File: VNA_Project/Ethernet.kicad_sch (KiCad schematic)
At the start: 0 parts

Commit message: minor changes eth
minor changes eth
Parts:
- added J1001: RJ45_Wuerth_7499010211A, Connector_RJ:RJ45_Wuerth_7499010211A_Horizontal, symbol Connector:RJ45_Wuerth_7499010211A
- added U1001: DP83848C, Package_QFP:LQFP-48_7x7mm_P0.5mm, symbol Interface_Ethernet:DP83848C
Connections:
- new net +3.3V: U1001.32 (IOVDD33), U1001.48 (IOVDD33)
- new net +3.3VA: U1001.22 (AVDD33)
- new net ETH_CRS_DV: U1001.40 (CRS/CRS_DV/LED_CFG)
- new net ETH_MDIO: U1001.30 (MDIO)
- new net ETH_RXD0: U1001.43 (RXD_0/PHY_AD1)
- new net ETH_RXD1: U1001.44 (RXD_1/PHY_AD2)
- new net ETH_RX_CLK: U1001.38 (RX_CLK)
- new net ETH_TXD0: U1001.3 (TXD_0)
- new net ETH_TXD1: U1001.4 (TXD_1)
- new net ETH_TX_EN: U1001.2 (TX_EN)
- new net GND: U1001.15 (AGND), U1001.19 (AGND), U1001.35 (IOGND), U1001.36 (DGND), U1001.47 (IOGND)
- new net NRST: U1001.29 (~{RESET})

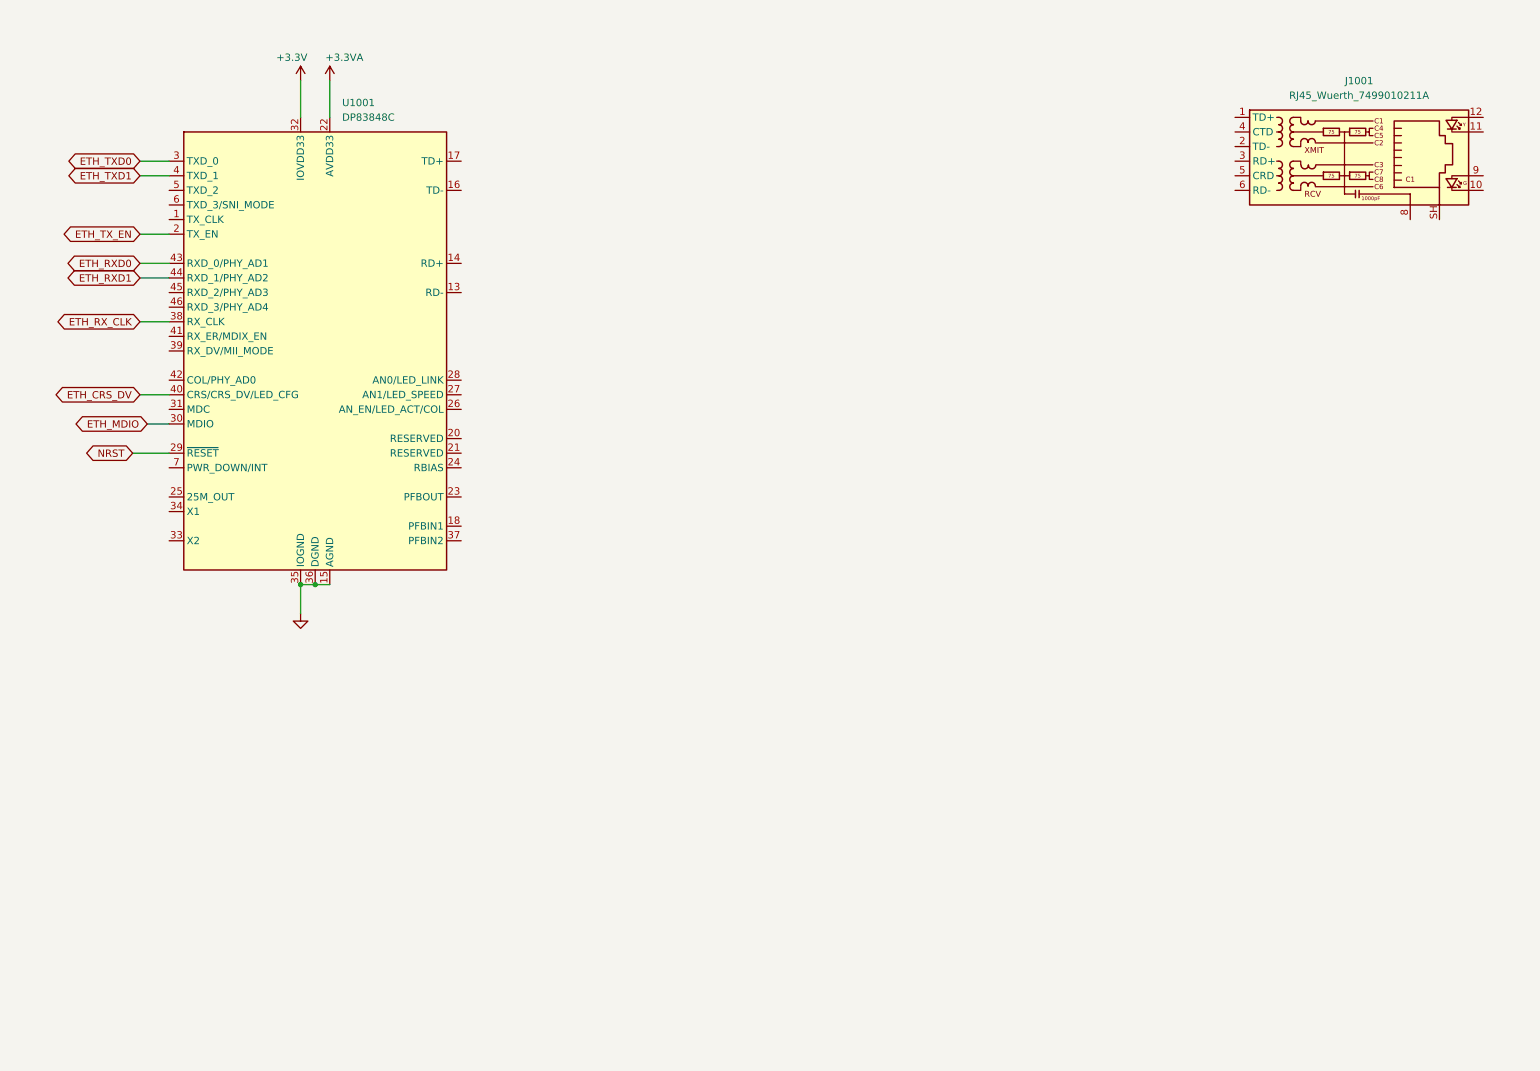
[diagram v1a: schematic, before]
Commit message: eth
eth
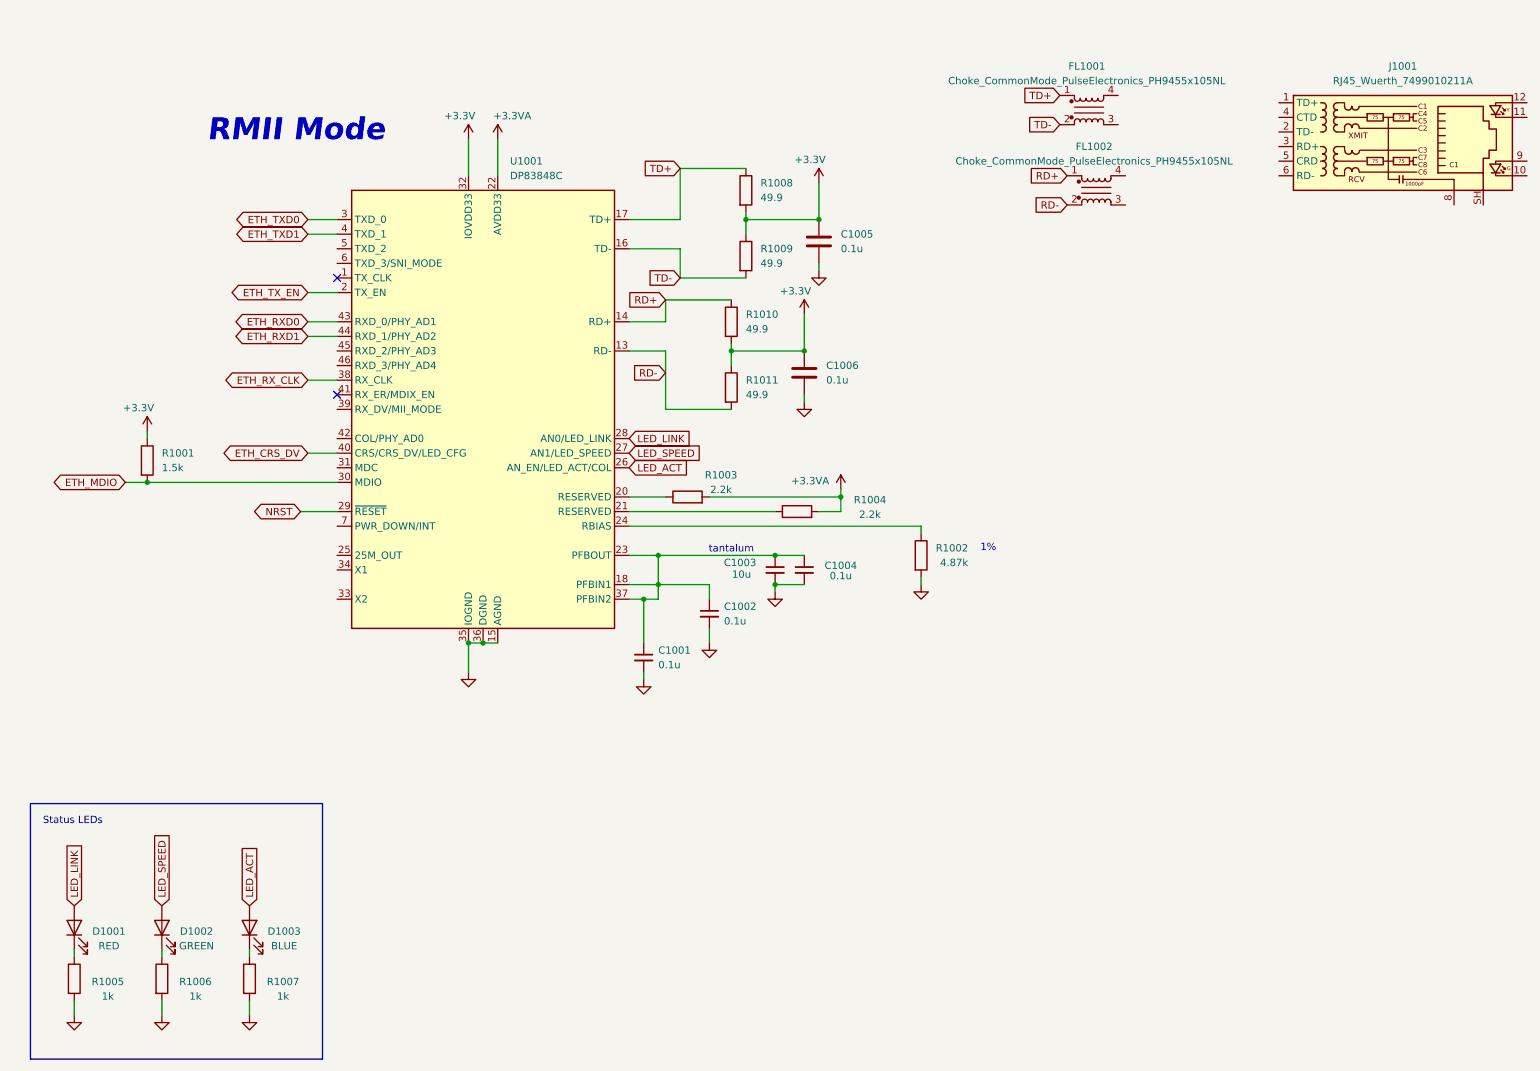
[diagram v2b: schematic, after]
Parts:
- added C1001, C1002, C1004: 0.1u, symbol Device:C_Small
- added C1003: 10u, symbol Device:C_Small
- added C1005, C1006: 0.1u, symbol Device:C
- added D1001: RED, symbol Device:LED
- added D1002: GREEN, symbol Device:LED
- added D1003: BLUE, symbol Device:LED
- added FL1001, FL1002: Choke_CommonMode_PulseElectronics_PH9455x105NL, Inductor_THT:L_CommonMode_PulseElectronics_PH9455x105NL_1, symbol Filter:Choke_CommonMode_PulseElectronics_PH9455x105NL
- added R1001: 1.5k, symbol Device:R
- added R1002: 4.87k, symbol Device:R
- added R1003, R1004: 2.2k, symbol Device:R
- added R1005, R1006, R1007: 1k, symbol Device:R
- added R1008, R1009, R1010, R1011: 49.9, symbol Device:R
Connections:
- net +3.3V: now also C1005.1, C1006.1, R1001.1, R1008.2, R1009.1, R1010.2, R1011.1
- net +3.3VA: now also R1003.2, R1004.2
- net ETH_MDIO: now also R1001.2
- net GND: now also C1001.2, C1002.2, C1003.2, C1004.2, C1005.2, C1006.2, R1002.2, R1005.2, R1006.2, R1007.2
- net RD-: now reaches U1001.13 (RD-)
- net RD-: now also FL1002.2, R1011.2
- net RD+: now reaches U1001.14 (RD+)
- net RD+: now also FL1002.1, R1010.1
- net TD-: now reaches U1001.16 (TD-)
- net TD-: now also FL1001.2, R1009.2
- net TD+: now reaches U1001.17 (TD+)
- net TD+: now also FL1001.1, R1008.1
- net at U1001.18 (PFBIN1): now also U1001.23 (PFBOUT), U1001.37 (PFBIN2), C1001.1, C1002.1, C1003.1, C1004.1
- net at U1001.20 (RESERVED): now also R1003.1
- net at U1001.21 (RESERVED): now also R1004.1
- net at U1001.24 (RBIAS): now also R1002.1
- net LED_ACT: now reaches U1001.26 (AN_EN/LED_ACT/COL)
- net LED_ACT: now also D1003.2 (A)
- net LED_SPEED: now reaches U1001.27 (AN1/LED_SPEED)
- net LED_SPEED: now also D1002.2 (A)
- net LED_LINK: now reaches U1001.28 (AN0/LED_LINK)
- net LED_LINK: now also D1001.2 (A)
- new net: D1001.1 (K), R1005.1
- new net: D1002.1 (K), R1006.1
- new net: D1003.1 (K), R1007.1
- no-connect marks 0 -> 2
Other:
- note added: "1%"
- note added: "RMII Mode"
- note added: "Status LEDs"
- note added: "tantalum"
- moved on the sheet: J1001, U1001

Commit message: Eth done
Eth done
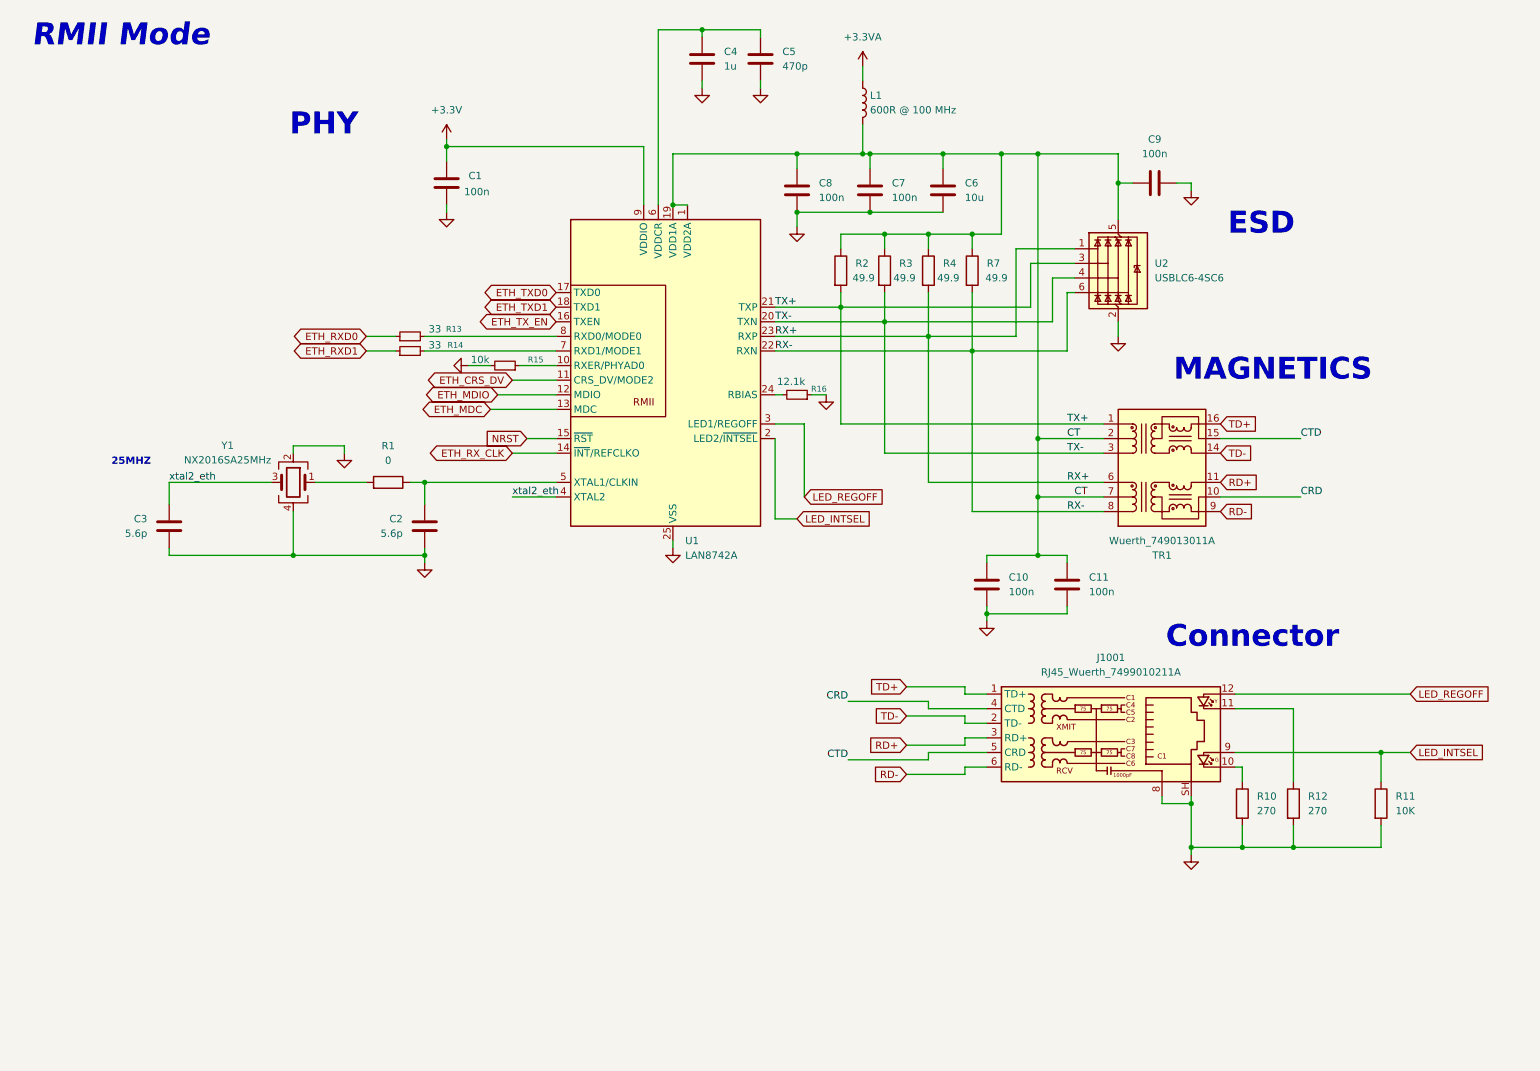
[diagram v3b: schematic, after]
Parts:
- removed C1001, C1002, C1004: 0.1u, symbol Device:C_Small
- removed C1003: 10u, symbol Device:C_Small
- removed C1005, C1006: 0.1u, symbol Device:C
- removed D1001: RED, symbol Device:LED
- removed D1002: GREEN, symbol Device:LED
- removed D1003: BLUE, symbol Device:LED
- removed FL1001, FL1002: Choke_CommonMode_PulseElectronics_PH9455x105NL, Inductor_THT:L_CommonMode_PulseElectronics_PH9455x105NL_1, symbol Filter:Choke_CommonMode_PulseElectronics_PH9455x105NL
- removed R1001: 1.5k, symbol Device:R
- removed R1002: 4.87k, symbol Device:R
- removed R1003, R1004: 2.2k, symbol Device:R
- removed R1005, R1006, R1007: 1k, symbol Device:R
- removed R1008, R1009, R1010, R1011: 49.9, symbol Device:R
- removed U1001: DP83848C, Package_QFP:LQFP-48_7x7mm_P0.5mm, symbol Interface_Ethernet:DP83848C
- added C1, C10, C11, C7, C8, C9: 100n, symbol Device:C
- added C2, C3: 5.6p, symbol Device:C
- added C4: 1u, symbol Device:C
- added C5: 470p, symbol Device:C
- added C6: 10u, symbol Device:C
- added L1: 600R @ 100 MHz, symbol Device:L
- added R1: 0, symbol Device:R
- added R10, R12: 270, symbol Device:R
- added R11: 10K, symbol Device:R
- added R13, R14: 33, symbol Device:R_Small
- added R15: 10k, symbol Device:R_Small
- added R16: 12.1k, symbol Device:R_Small
- added R2, R3, R4, R7: 49.9, symbol Device:R
- added TR1: Wuerth_749013011A, Transformer_SMD:Transformer_Ethernet_Wuerth_749013011A, symbol Transformer:Wuerth_749013011A
- added U1: LAN8742A, Package_DFN_QFN:VQFN-24-1EP_4x4mm_P0.5mm_EP2.5x2.5mm_ThermalVias, symbol Interface_Ethernet:LAN8742A
- added U2: USBLC6-4SC6, Package_TO_SOT_SMD:SOT-23-6, symbol Power_Protection:USBLC6-4SC6
- added Y1: NX2016SA25MHz, symbol Device:Crystal_GND24
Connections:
- net +3.3V: now also C1.1, U1.9 (VDDIO)
- net +3.3VA: now also L1.1
- net ETH_CRS_DV: now also U1.11 (CRS_DV/MODE2)
- net ETH_MDIO: now also U1.12 (MDIO)
- net ETH_RXD0: now also R13.1
- net ETH_RXD1: now also R14.1
- net ETH_RX_CLK: now also U1.14 (~{INT}/REFCLKO)
- net ETH_TXD0: now also U1.17 (TXD0)
- net ETH_TXD1: now also U1.18 (TXD1)
- net ETH_TX_EN: now also U1.16 (TXEN)
- net GND: now also J1001.8, J1001.SH, C1.2, C10.2, C11.2, C2.2, C3.2, C4.2, C5.2, C6.2, C7.2, C8.2, C9.2, R10.2, R11.2, R12.2, R15.2, R16.1, U1.25 (VSS), U2.2 (GND), Y1.2, Y1.4
- net NRST: now also U1.15 (~{RST})
- net RD+: now also J1001.3 (RD+), TR1.11 (RX+)
- net RD-: now also J1001.6 (RD-), TR1.9 (RX-)
- net TD+: now also J1001.1 (TD+), TR1.16 (TX+)
- net TD-: now also J1001.2 (TD-), TR1.14 (TX-)
- net at J1001.10: now also R10.1
- net at J1001.11: now also R12.1
- net LED_REGOFF: now reaches J1001.12
- net LED_REGOFF: now also U1.3 (LED1/REGOFF)
- net CRD: now reaches J1001.4 (CTD)
- net CRD: now also TR1.10 (C_RX)
- net CTD: now reaches J1001.5 (CRD)
- net CTD: now also TR1.15 (C_TX)
- net LED_INTSEL: now reaches J1001.9
- net LED_INTSEL: now also R11.1, U1.2 (LED2/~{INTSEL})
- new net: R13.2, U1.8 (RXD0/MODE0)
- new net: R15.1, U1.10 (RXER/PHYAD0)
- new net: R16.2, U1.24 (RBIAS)
- new net: C2.1, R1.1, U1.5 (XTAL1/CLKIN)
- new net: C4.1, C5.1, U1.6 (VDDCR)
- new net: R14.2, U1.7 (RXD1/MODE1)
- new net: R1.2, Y1.1
- new net CT: C10.1, C11.1, C6.1, C7.1, C8.1, C9.1, L1.2, R2.1, R3.1, R4.1, R7.1, TR1.2 (C_TD), TR1.7 (C_RD), U1.1 (VDD2A), U1.19 (VDD1A), U2.5 (VBUS)
- new net ETH_MDC: U1.13 (MDC)
- new net RX+: R4.2, TR1.6 (RD+), U1.23 (RXP), U2.1 (I/O1)
- new net RX-: R7.2, TR1.8 (RD-), U1.22 (RXN), U2.6 (I/O4)
- new net TX+: R2.2, TR1.1 (TD+), U1.21 (TXP), U2.3 (I/O2)
- new net TX-: R3.2, TR1.3 (TD-), U1.20 (TXN), U2.4 (I/O3)
- new net xtal2_eth: C3.1, U1.4 (XTAL2), Y1.3
- no-connect marks 2 -> 0
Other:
- note added: "25MHZ"
- note added: "Connector"
- note added: "ESD"
- note added: "MAGNETICS"
- note added: "PHY"
- note removed: "1%"
- note removed: "Status LEDs"
- note removed: "tantalum"
- moved on the sheet: J1001
